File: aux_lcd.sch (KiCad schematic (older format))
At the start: 12 parts, among them P1 DEBUG, P2 LCD, U1 ADXL362

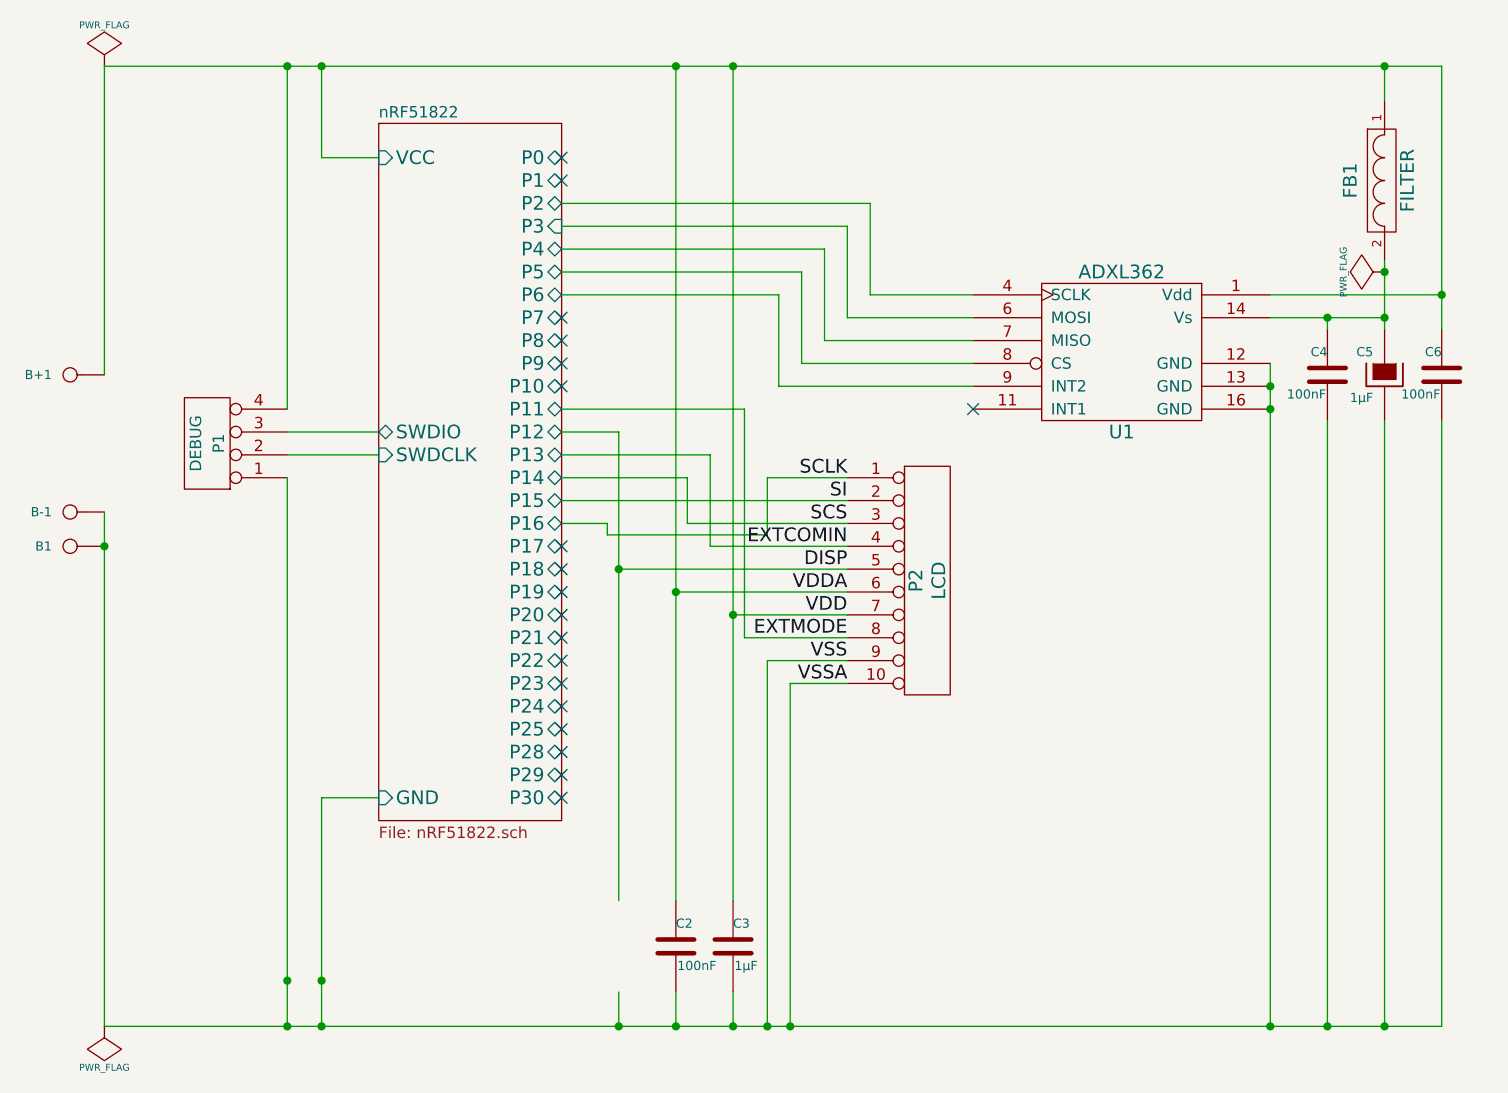
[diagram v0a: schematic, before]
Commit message: 0.0.2
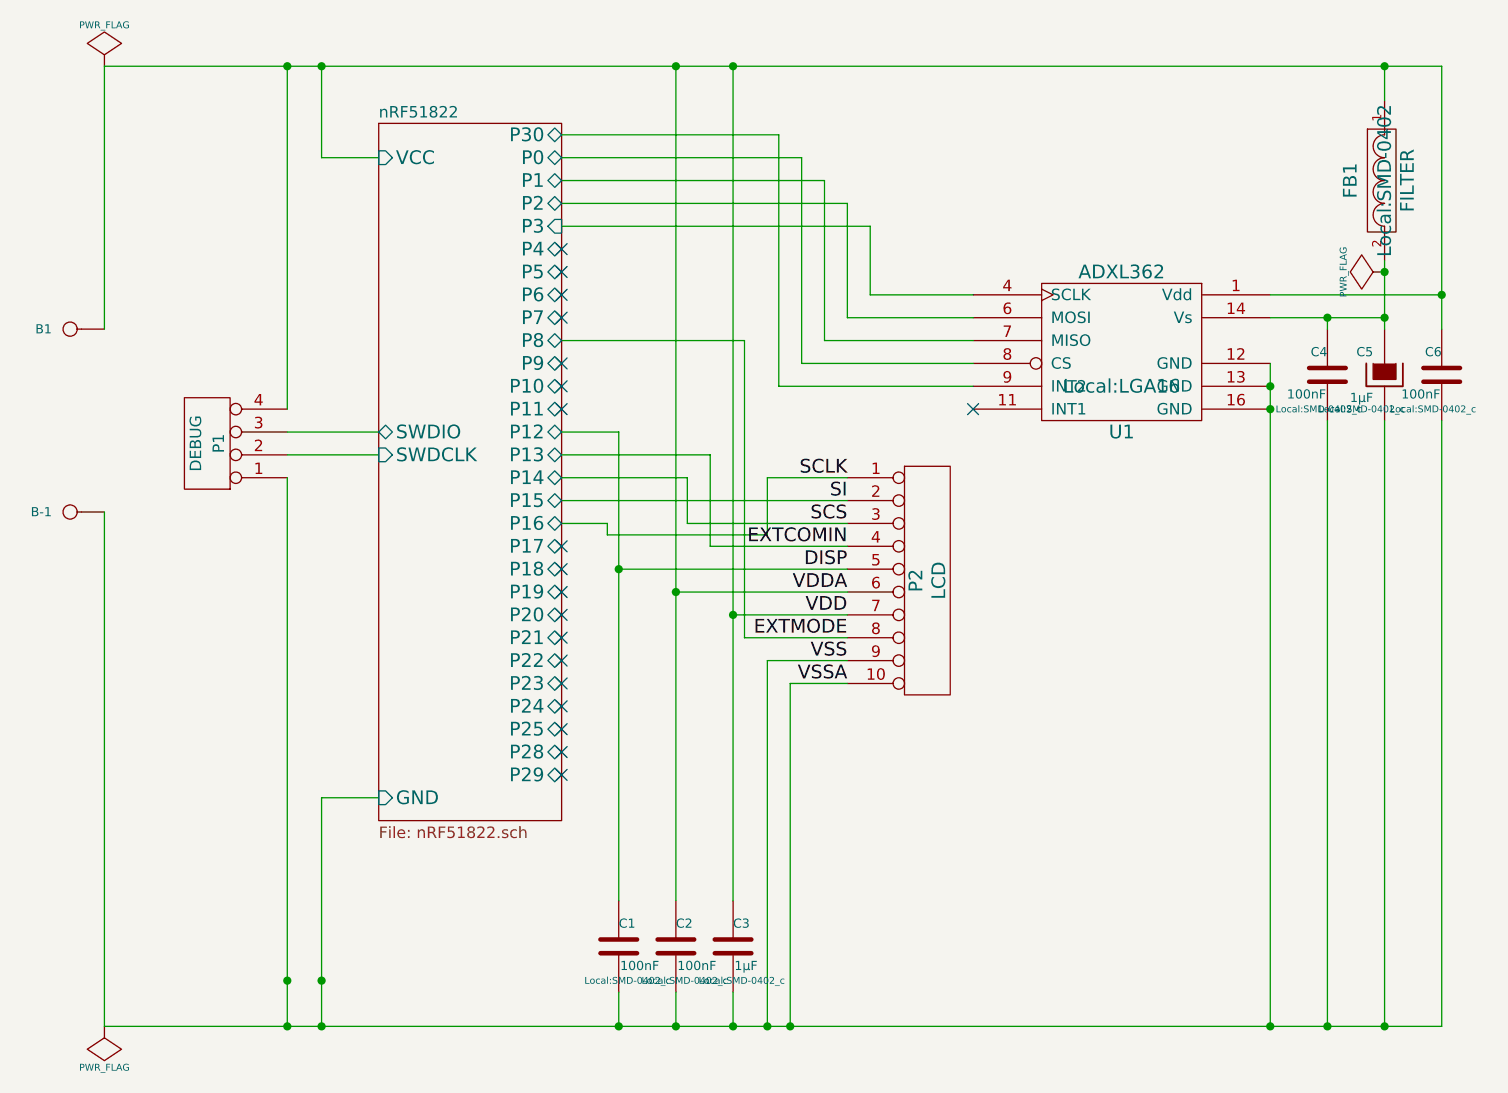
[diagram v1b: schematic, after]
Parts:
- removed B+1: CONN_1, symbol CONN_1
- added C1: 100nF, Local:SMD-0402_c, symbol C
- B-1: footprint (none) -> Connect:SIL-1
- B1: footprint (none) -> Local:CR2032
- C2, C3, C4, C5, C6: footprint ~ -> Local:SMD-0402_c
- FB1: footprint ~ -> Local:SMD-0402
- P1: footprint (none) -> Local:4-PIN-1.27mm
- P2: footprint (none) -> Local:FPC10
- U1: footprint ~ -> Local:LGA16
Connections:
- net DISP: now also C1.1
- net VDD: now also B1.1
- net VSS: now also C1.2; no longer B1.1
- net nRF51822/P0: now also U1.8 (CS)
- net nRF51822/P1: now also U1.7 (MISO)
- net nRF51822/P2: now also U1.6 (MOSI); no longer U1.4 (SCLK)
- net nRF51822/P3: now also U1.4 (SCLK); no longer U1.6 (MOSI)
- net nRF51822/P30: now also U1.9 (INT2)
- net nRF51822/P4: no longer U1.7 (MISO)
- net nRF51822/P5: no longer U1.8 (CS)
- net nRF51822/P6: no longer U1.9 (INT2)
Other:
- moved on the sheet: B1
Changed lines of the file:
@@
 LIBS:adxl362
 LIBS:aux_lcd-cache
-EELAYER 27 0
+EELAYER 24 0
 EELAYER END
 $Descr A4 11693 8268
@@
 F30 "P28" B R 4650 4750 60
 F31 "P29" B R 4650 4850 60
-F32 "P30" B R 4650 4950 60
+F32 "P30" B R 4650 2050 60
 F33 "VCC" I L 3850 2150 60
 F34 "GND" I L 3850 4950 60
@@
 F 0 "P2" V 6200 4000 60  0000 C CNN
 F 1 "LCD" V 6300 4000 60  0000 C CNN
-F 2 "" H 6250 4000 60  0000 C CNN
+F 2 "Local:FPC10" H 6250 4000 60  0001 C CNN
 F 3 "" H 6250 4000 60  0000 C CNN
 	1    6250 4000
@@
 F 0 "C2" H 5150 5700 40  0000 L CNN
 F 1 "100nF" H 5156 5515 40  0000 L CNN
-F 2 "~" H 5188 5450 30  0000 C CNN
+F 2 "Local:SMD-0402_c" H 5188 5450 30  0000 C CNN
 F 3 "~" H 5150 5600 60  0000 C CNN
 	1    5150 5600
@@
 F 0 "C3" H 5400 5700 40  0000 L CNN
 F 1 "1µF" H 5406 5515 40  0000 L CNN
-F 2 "~" H 5438 5450 30  0000 C CNN
+F 2 "Local:SMD-0402_c" H 5438 5450 30  0000 C CNN
 F 3 "~" H 5400 5600 60  0000 C CNN
 	1    5400 5600
@@
 F 0 "U1" H 7100 2650 60  0000 C CNN
 F 1 "ADXL362" H 7100 3350 60  0000 C CNN
-F 2 "~" H 7100 2850 60  0000 C CNN
+F 2 "Local:LGA16" H 7100 2850 60  0000 C CNN
 F 3 "~" H 7100 2850 60  0000 C CNN
 	1    7100 3000
@@
 F 0 "C4" H 8000 3200 40  0000 L CNN
 F 1 "100nF" H 8006 3015 40  0000 L CNN
-F 2 "~" H 8038 2950 30  0000 C CNN
+F 2 "Local:SMD-0402_c" H 8038 2950 30  0000 C CNN
 F 3 "~" H 8000 3100 60  0000 C CNN
 	1    8000 3100
@@
 F 0 "C5" H 8300 3200 40  0000 L CNN
 F 1 "1µF" H 8300 3000 40  0000 L CNN
-F 2 "~" H 8350 2950 30  0000 C CNN
+F 2 "Local:SMD-0402_c" H 8350 2950 30  0000 C CNN
 F 3 "~" H 8250 3100 300 0000 C CNN
 	1    8250 3100
@@
 F 0 "FB1" H 8250 2400 60  0000 C CNN
 F 1 "FILTER" H 8250 2150 60  0000 C CNN
-F 2 "~" H 8250 2250 60  0000 C CNN
+F 2 "Local:SMD-0402" H 8250 2250 60  0000 C CNN
 F 3 "~" H 8250 2250 60  0000 C CNN
 	1    8250 2250
@@
 F 0 "C6" H 8500 3200 40  0000 L CNN
 F 1 "100nF" H 8506 3015 40  0000 L CNN
-F 2 "~" H 8538 2950 30  0000 C CNN
+F 2 "Local:SMD-0402_c" H 8538 2950 30  0000 C CNN
 F 3 "~" H 8500 3100 60  0000 C CNN
 	1    8500 3100
@@
 F 0 "P1" V 3050 3400 50  0000 C CNN
 F 1 "DEBUG" V 3150 3400 50  0000 C CNN
-F 2 "" H 3100 3400 60  0000 C CNN
+F 2 "Local:4-PIN-1.27mm" H 3100 3400 60  0001 C CNN
 F 3 "" H 3100 3400 60  0000 C CNN
 	1    3100 3400
 	-1   0    0    1
 $EndComp
-NoConn ~ 4650 2150
-NoConn ~ 4650 2250
+$Comp
+L PWR_FLAG #FLG1
+U 1 1 532A11CD
+P 2650 1750
+F 0 "#FLG1" H 2650 1845 30  0001 C CNN
+F 1 "PWR_FLAG" H 2650 1930 30  0000 C CNN
+F 2 "" H 2650 1750 60  0000 C CNN
+F 3 "" H 2650 1750 60  0000 C CNN
+	1    2650 1750
+	1    0    0    -1
+$EndComp
+$Comp
+L PWR_FLAG #FLG2
+U 1 1 532A11DA
+P 2650 5950
+F 0 "#FLG2" H 2650 6045 30  0001 C CNN
+F 1 "PWR_FLAG" H 2650 6130 30  0000 C CNN
+F 2 "" H 2650 5950 60  0000 C CNN
+F 3 "" H 2650 5950 60  0000 C CNN
+	1    2650 5950
+	-1   0    0    1
+$EndComp
+$Comp
+L PWR_FLAG #FLG3
+U 1 1 532A1C24
+P 8250 2650
+F 0 "#FLG3" H 8250 2745 30  0001 C CNN
+F 1 "PWR_FLAG" H 8250 2830 30  0000 C CNN
+F 2 "" H 8250 2650 60  0000 C CNN
+F 3 "" H 8250 2650 60  0000 C CNN
+	1    8250 2650
+	0    -1   -1   0
+$EndComp
+NoConn ~ 4650 4450
+NoConn ~ 4650 4550
+NoConn ~ 4650 4650
+NoConn ~ 4650 4750
+NoConn ~ 4650 4850
+NoConn ~ 4650 3850
+NoConn ~ 4650 3950
+NoConn ~ 4650 4050
+NoConn ~ 4650 4150
+NoConn ~ 4650 4250
+NoConn ~ 4650 4350
+$Comp
+L CONN_1 B-1
+U 1 1 532B1687
+P 2500 3700
+F 0 "B-1" H 2580 3700 40  0000 L CNN
+F 1 "CONN_1" H 2500 3755 30  0001 C CNN
+F 2 "Connect:SIL-1" H 2500 3700 60  0001 C CNN
+F 3 "" H 2500 3700 60  0000 C CNN
+	1    2500 3700
+	-1   0    0    1
+$EndComp
+$Comp
+L CONN_1 B1
+U 1 1 532B6FEF
+P 2500 2900
+F 0 "B1" H 2580 2900 40  0000 L CNN
+F 1 "CONN_1" H 2500 2955 30  0001 C CNN
+F 2 "Local:CR2032" H 2500 2900 60  0001 C CNN
+F 3 "" H 2500 2900 60  0000 C CNN
+	1    2500 2900
+	-1   0    0    1
+$EndComp
+NoConn ~ 6450 3250
+NoConn ~ 4650 2850
+NoConn ~ 4650 3050
+NoConn ~ 4650 3250
+NoConn ~ 4650 3150
+$Comp
+L C C1
+U 1 1 53FF5DBB
+P 4900 5600
+F 0 "C1" H 4900 5700 40  0000 L CNN
+F 1 "100nF" H 4906 5515 40  0000 L CNN
+F 2 "Local:SMD-0402_c" H 4938 5450 30  0000 C CNN
+F 3 "~" H 4900 5600 60  0000 C CNN
+	1    4900 5600
+	1    0    0    -1
+$EndComp
+NoConn ~ 4650 2550
+NoConn ~ 4650 2650
+NoConn ~ 4650 2750
 Wire Wire Line
 	3600 2150 3850 2150
@@
 	8000 2900 8000 2850
 Connection ~ 8000 2850
-Wire Wire Line
-	2650 3100 2650 1750
 Wire Wire Line
 	3450 3550 3450 5950
@@
 	8500 5950 8500 3300
 Connection ~ 8250 5950
-$Comp
-L PWR_FLAG #FLG01
-U 1 1 532A11CD
-P 2650 1750
-F 0 "#FLG01" H 2650 1845 30  0001 C CNN
-F 1 "PWR_FLAG" H 2650 1930 30  0000 C CNN
-F 2 "" H 2650 1750 60  0000 C CNN
-F 3 "" H 2650 1750 60  0000 C CNN
-	1    2650 1750
-	1    0    0    -1
-$EndComp
-$Comp
-L PWR_FLAG #FLG02
-U 1 1 532A11DA
-P 2650 5950
-F 0 "#FLG02" H 2650 6045 30  0001 C CNN
-F 1 "PWR_FLAG" H 2650 6130 30  0000 C CNN
-F 2 "" H 2650 5950 60  0000 C CNN
-F 3 "" H 2650 5950 60  0000 C CNN
-	1    2650 5950
-	-1   0    0    1
-$EndComp
-$Comp
-L PWR_FLAG #FLG03
-U 1 1 532A1C24
-P 8250 2650
-F 0 "#FLG03" H 8250 2745 30  0001 C CNN
-F 1 "PWR_FLAG" H 8250 2830 30  0000 C CNN
-F 2 "" H 8250 2650 60  0000 C CNN
-F 3 "" H 8250 2650 60  0000 C CNN
-	1    8250 2650
-	0    -1   -1   0
-$EndComp
-NoConn ~ 4650 4450
-NoConn ~ 4650 4550
-NoConn ~ 4650 4650
-NoConn ~ 4650 4750
-NoConn ~ 4650 4850
-NoConn ~ 4650 4950
 Connection ~ 8250 2650
 Wire Wire Line
 	8250 1900 8250 1750
 Wire Wire Line
-	5900 4250 5450 4250
-Wire Wire Line
-	5450 4250 5450 3250
-Wire Wire Line
-	5450 3250 4650 3250
+	5450 4250 5900 4250
 Wire Wire Line
 	5900 3950 4900 3950
+Connection ~ 4900 3950
+Wire Wire Line
+	5900 3850 5300 3850
+Wire Wire Line
+	5300 3850 5300 3450
+Wire Wire Line
+	5300 3450 4650 3450
+Wire Wire Line
+	5900 3750 5200 3750
+Wire Wire Line
+	5200 3750 5200 3550
+Wire Wire Line
+	5200 3550 4650 3550
+Wire Wire Line
+	4650 3650 5900 3650
+Wire Wire Line
+	5900 3550 5550 3550
+Wire Wire Line
+	5550 3550 5550 3800
+Wire Wire Line
+	5550 3800 4850 3800
+Wire Wire Line
+	4850 3800 4850 3750
+Wire Wire Line
+	4850 3750 4650 3750
+Wire Wire Line
+	5600 3150 6450 3150
+Wire Wire Line
+	5600 2050 5600 3150
+Wire Wire Line
+	5700 3050 6450 3050
+Wire Wire Line
+	5700 2150 5700 3050
+Wire Wire Line
+	5800 2950 6450 2950
+Wire Wire Line
+	5800 2250 5800 2950
+Wire Wire Line
+	5900 2850 6450 2850
+Wire Wire Line
+	5900 2350 5900 2850
+Wire Wire Line
+	6450 2750 6000 2750
+Wire Wire Line
+	2650 2900 2650 1750
+Wire Wire Line
+	5600 2050 4650 2050
+Wire Wire Line
+	4650 2150 5700 2150
+Wire Wire Line
+	4650 2250 5800 2250
+Wire Wire Line
+	4650 2350 5900 2350
+Wire Wire Line
+	4650 2450 6000 2450
+Wire Wire Line
+	6000 2450 6000 2750
+Wire Wire Line
+	5450 2950 5450 4250
+Wire Wire Line
+	4900 3350 4900 5400
 Wire Wire Line
 	4900 3350 4650 3350
-Connection ~ 4900 3950
-Wire Wire Line
-	5900 3850 5300 3850
-Wire Wire Line
-	5300 3850 5300 3450
-Wire Wire Line
-	5300 3450 4650 3450
-Wire Wire Line
-	5900 3750 5200 3750
-Wire Wire Line
-	5200 3750 5200 3550
-Wire Wire Line
-	5200 3550 4650 3550
-Wire Wire Line
-	4650 3650 5900 3650
-Wire Wire Line
-	5900 3550 5550 3550
-Wire Wire Line
-	5550 3550 5550 3800
-Wire Wire Line
-	5550 3800 4850 3800
-Wire Wire Line
-	4850 3800 4850 3750
-Wire Wire Line
-	4850 3750 4650 3750
-NoConn ~ 4650 3850
-NoConn ~ 4650 3950
-NoConn ~ 4650 4050
-NoConn ~ 4650 4150
-NoConn ~ 4650 4250
-NoConn ~ 4650 4350
-Wire Wire Line
-	6450 3150 5600 3150
-Wire Wire Line
-	5600 3150 5600 2750
-Wire Wire Line
-	5600 2750 4650 2750
-Wire Wire Line
-	6450 3050 5700 3050
-Wire Wire Line
-	5700 3050 5700 2650
-Wire Wire Line
-	5700 2650 4650 2650
-Wire Wire Line
-	6450 2950 5800 2950
-Wire Wire Line
-	5800 2950 5800 2550
-Wire Wire Line
-	5800 2550 4650 2550
-Wire Wire Line
-	6450 2850 5900 2850
-Wire Wire Line
-	5900 2850 5900 2450
-Wire Wire Line
-	5900 2450 4650 2450
-Wire Wire Line
-	6450 2750 6000 2750
-Wire Wire Line
-	6000 2750 6000 2350
-Wire Wire Line
-	6000 2350 4650 2350
-$Comp
-L CONN_1 B+1
-U 1 1 532B167A
-P 2500 3100
-F 0 "B+1" H 2580 3100 40  0000 L CNN
-F 1 "CONN_1" H 2500 3155 30  0001 C CNN
-F 2 "" H 2500 3100 60  0000 C CNN
-F 3 "" H 2500 3100 60  0000 C CNN
-	1    2500 3100
-	-1   0    0    1
-$EndComp
-$Comp
-L CONN_1 B-1
-U 1 1 532B1687
-P 2500 3700
-F 0 "B-1" H 2580 3700 40  0000 L CNN
-F 1 "CONN_1" H 2500 3755 30  0001 C CNN
-F 2 "" H 2500 3700 60  0000 C CNN
-F 3 "" H 2500 3700 60  0000 C CNN
-	1    2500 3700
-	-1   0    0    1
-$EndComp
-$Comp
-L CONN_1 B1
-U 1 1 532B6FEF
-P 2500 3850
-F 0 "B1" H 2580 3850 40  0000 L CNN
-F 1 "CONN_1" H 2500 3905 30  0001 C CNN
-F 2 "" H 2500 3850 60  0000 C CNN
-F 3 "" H 2500 3850 60  0000 C CNN
-	1    2500 3850
-	-1   0    0    1
-$EndComp
-Connection ~ 2650 3850
-NoConn ~ 6450 3250
-NoConn ~ 4650 2850
-Wire Wire Line
-	4900 3350 4900 5400
-NoConn ~ 4650 2950
-NoConn ~ 4650 3050
-NoConn ~ 4650 3150
+Wire Wire Line
+	4650 2950 5450 2950
 $EndSCHEMATC
